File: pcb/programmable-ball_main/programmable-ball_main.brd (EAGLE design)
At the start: 30.5 x 30.8 mm, 2 parts, among them J1 USB4125-GF-A_REVA2, U1 MDBT50Q-1MV2

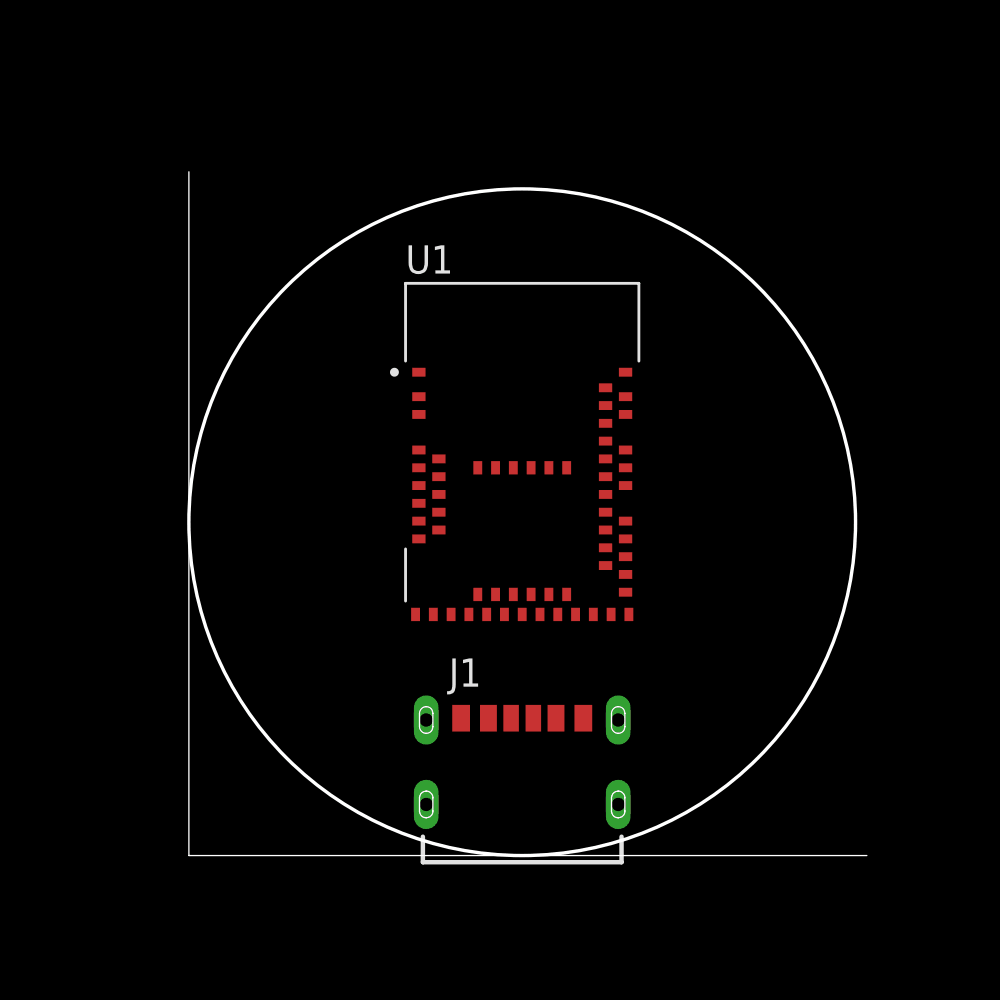
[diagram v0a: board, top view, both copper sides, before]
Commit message: 軽微な修正
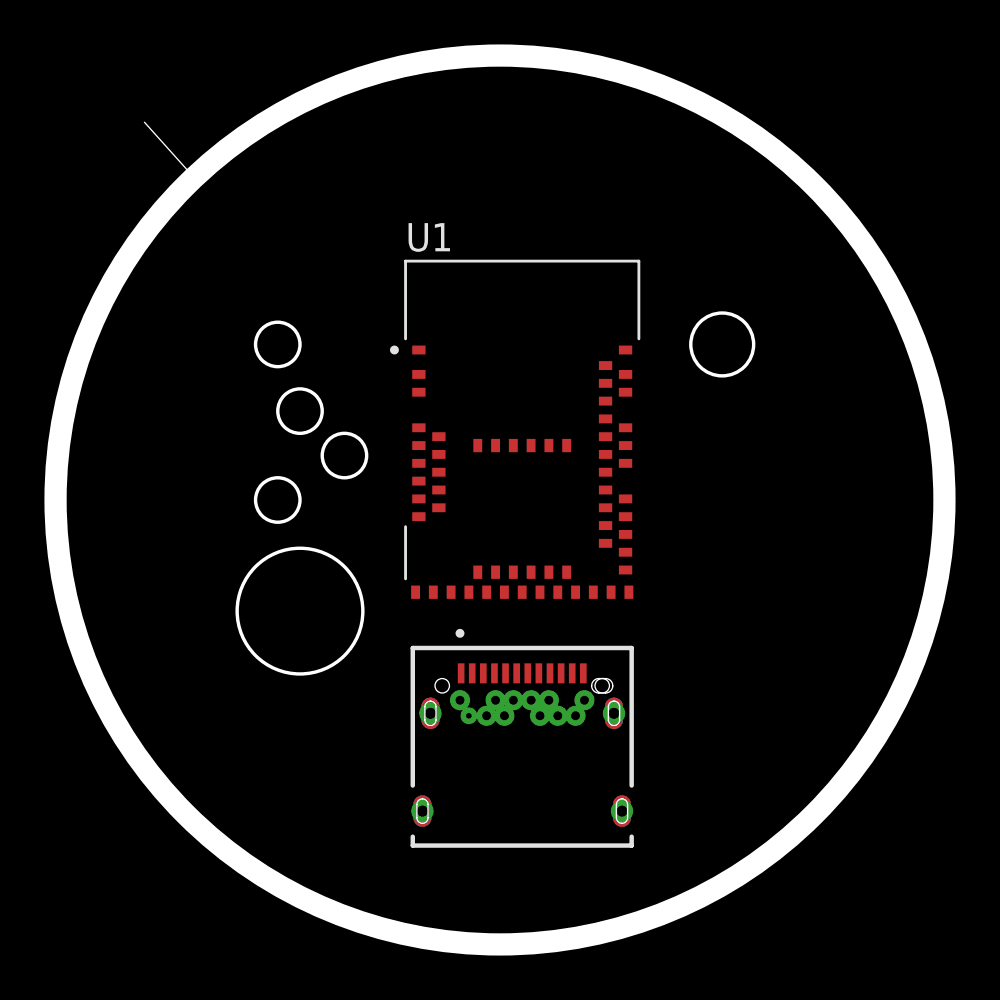
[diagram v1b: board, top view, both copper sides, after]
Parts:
- J1: value USB4125-GF-A_REVA2 -> USB4056-03-A_REVA2; device USB4125-GF-A_REVA2:GCT_USB4125-GF-A_REVA2 -> USB4056-03-A_REVA2:GCT_USB4056-03-A_REVA2
- moved J1 1.10 mm to (15.0, 2.00)
- moved U1 1.00 mm to (15.0, 19.0)
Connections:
- new net GND_A: J1.A1, J1.A12
- new net GND_B: J1.B1, J1.B12
- new net SHELL_GND: J1.S1, J1.S2, J1.S3, J1.S4
- new net USBD+: U1.35
- new net USBD-: U1.34
- new net VBUS_A: J1.A4, J1.A9
- new net VBUS_B: J1.B4, J1.B9
- net GND: no longer J1.A12, J1.B12
- net VBUS: no longer J1.A9, J1.B9
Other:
- board size 30.5 x 30.8 mm -> 40 x 40 mm
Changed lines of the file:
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@@
 <board>
 <plain>
-<wire x1="0" y1="0" x2="30.51" y2="0" width="0" layer="20"/>
-<wire x1="0" y1="30.77" x2="0" y2="0" width="0" layer="20"/>
+<wire x1="0" y1="30.77" x2="-2" y2="33" width="0" layer="20"/>
 <dimension x1="0" y1="0" x2="0" y2="30" x3="-6" y3="15" textsize="1.778" layer="47"/>
 <dimension x1="0" y1="0" x2="30" y2="0" x3="15" y3="-6" textsize="1.778" layer="47"/>
-<circle x="15" y="15" radius="15" width="0.1524" layer="20"/>
+<circle x="14" y="16" radius="20" width="1" layer="20"/>
+<circle x="4" y="16" radius="1" width="0.1524" layer="20"/>
+<circle x="5" y="11" radius="2.828425" width="0.1524" layer="20"/>
+<circle x="7" y="18" radius="1" width="0.1524" layer="20"/>
+<circle x="4" y="23" radius="1" width="0.1524" layer="20"/>
+<circle x="5" y="20" radius="1" width="0.1524" layer="20"/>
+<circle x="24" y="23" radius="1.4142125" width="0.1524" layer="20"/>
 </plain>
 <attributes>
@@
 </autorouter>
 <elements>
-<element name="U1" library="MDBT50Q-1MV2" package="XCVR_MDBT50Q-1MV2" value="MDBT50Q-1MV2" x="15" y="18" smashed="yes">
-<attribute name="AVAILABILITY" value="In Stock" x="15" y="18" size="1.778" layer="27" display="off"/>
-<attribute name="CHECK_PRICES" value="https://www.snapeda.com/parts/MDBT50Q-1MV2/Raytac+Corporation/view-part/?ref=eda" x="15" y="18" size="1.778" layer="27" display="off"/>
-<attribute name="DESCRIPTION" value=" 802.15.4, Bluetooth Bluetooth v5.2, Zigbee® Transceiver Module 2.36GHz ~ 2.5GHz Integrated, Chip Surface Mount " x="15" y="18" size="1.778" layer="27" display="off"/>
-<attribute name="MF" value="Raytac Corporation" x="15" y="18" size="1.778" layer="27" display="off"/>
-<attribute name="MP" value="MDBT50Q-1MV2" x="15" y="18" size="1.778" layer="27" display="off"/>
-<attribute name="NAME" x="9.75" y="26.19" size="1.27" layer="25"/>
-<attribute name="PACKAGE" value="SMD-61 Raytac Corporation" x="15" y="18" size="1.778" layer="27" display="off"/>
-<attribute name="PRICE" value="None" x="15" y="18" size="1.778" layer="27" display="off"/>
-<attribute name="SNAPEDA_LINK" value="https://www.snapeda.com/parts/MDBT50Q-1MV2/Raytac+Corporation/view-part/?ref=snap" x="15" y="18" size="1.778" layer="27" display="off"/>
+<element name="U1" library="MDBT50Q-1MV2" package="XCVR_MDBT50Q-1MV2" value="MDBT50Q-1MV2" x="15" y="19" smashed="yes">
+<attribute name="AVAILABILITY" value="In Stock" x="15" y="19" size="1.778" layer="27" display="off"/>
+<attribute name="CHECK_PRICES" value="https://www.snapeda.com/parts/MDBT50Q-1MV2/Raytac+Corporation/view-part/?ref=eda" x="15" y="19" size="1.778" layer="27" display="off"/>
+<attribute name="DESCRIPTION" value=" 802.15.4, Bluetooth Bluetooth v5.2, Zigbee® Transceiver Module 2.36GHz ~ 2.5GHz Integrated, Chip Surface Mount " x="15" y="19" size="1.778" layer="27" display="off"/>
+<attribute name="MF" value="Raytac Corporation" x="15" y="19" size="1.778" layer="27" display="off"/>
+<attribute name="MP" value="MDBT50Q-1MV2" x="15" y="19" size="1.778" layer="27" display="off"/>
+<attribute name="NAME" x="9.75" y="27.19" size="1.27" layer="25"/>
+<attribute name="PACKAGE" value="SMD-61 Raytac Corporation" x="15" y="19" size="1.778" layer="27" display="off"/>
+<attribute name="PRICE" value="None" x="15" y="19" size="1.778" layer="27" display="off"/>
+<attribute name="SNAPEDA_LINK" value="https://www.snapeda.com/parts/MDBT50Q-1MV2/Raytac+Corporation/view-part/?ref=snap" x="15" y="19" size="1.778" layer="27" display="off"/>
 </element>
-<element name="J1" library="USB4125-GF-A_REVA2" package="GCT_USB4125-GF-A_REVA2" value="USB4125-GF-A_REVA2" x="15" y="3.1" smashed="yes">
-<attribute name="DESCRIPTION" value=" USB Charge Only Connector Type C Horizontal Receptacle, 3.16mm profile, 6 Pins, Surface mount, Top mount, low cost " x="15" y="3.1" size="1.778" layer="27" display="off"/>
-<attribute name="DIGI-KEY_PART_NUMBER" value="2073-USB4125-GF-ATR-ND" x="15" y="3.1" size="1.778" layer="27" display="off"/>
-<attribute name="MF" value="Global Connector Technology" x="15" y="3.1" size="1.778" layer="27" display="off"/>
-<attribute name="MP" value="USB4125-GF-A" x="15" y="3.1" size="1.778" layer="27" display="off"/>
-<attribute name="NAME" x="11.7" y="7.6" size="1.27" layer="25"/>
-<attribute name="PACKAGE" value="None" x="15" y="3.1" size="1.778" layer="27" display="off"/>
-<attribute name="PURCHASE-URL" value="https://pricing.snapeda.com/search/part/USB4125-GF-A/?ref=eda" x="15" y="3.1" size="1.778" layer="27" display="off"/>
+<element name="J1" library="USB4056-03-A_REVA2" package="GCT_USB4056-03-A_REVA2" value="USB4056-03-A_REVA2" x="15" y="2" smashed="yes">
+<attribute name="AVAILABILITY" value="In Stock" x="15" y="2" size="1.778" layer="27" display="off"/>
+<attribute name="CHECK_PRICES" value="https://www.snapeda.com/parts/USB4056-03-A/Global+Connector+Technology/view-part/?ref=eda" x="15" y="2" size="1.778" layer="27" display="off"/>
+<attribute name="DESCRIPTION" value=" USB-C (USB TYPE-C) USB 3.2 Gen 2 (USB 3.1 Gen 2, Superspeed + (USB 3.1)) Receptacle Connector 24 Position Surface Mount, Right Angle; Through Hole " x="15" y="2" size="1.778" layer="27" display="off"/>
+<attribute name="MF" value="Global Connector Technology" x="15" y="2" size="1.778" layer="27" display="off"/>
+<attribute name="MP" value="USB4056-03-A" x="15" y="2" size="1.778" layer="27" display="off"/>
+<attribute name="PACKAGE" value="None" x="15" y="2" size="1.778" layer="27" display="off"/>
+<attribute name="PRICE" value="None" x="15" y="2" size="1.778" layer="27" display="off"/>
+<attribute name="SNAPEDA_LINK" value="https://www.snapeda.com/parts/USB4056-03-A/Global+Connector+Technology/view-part/?ref=snap" x="15" y="2" size="1.778" layer="27" display="off"/>
 </element>
 </elements>
@@
 <contactref element="U1" pad="33"/>
 <contactref element="U1" pad="2"/>
-<contactref element="J1" pad="B12"/>
-<contactref element="J1" pad="A12"/>
-<wire x1="10.35" y1="21.75" x2="19.65" y2="21.75" width="0" layer="19" extent="1-1"/>
-<wire x1="10.35" y1="20.65" x2="10.35" y2="21.75" width="0" layer="19" extent="1-1"/>
-<wire x1="10.2" y1="10.85" x2="10.35" y2="20.65" width="0" layer="19" extent="1-1"/>
-<wire x1="19.8" y1="10.85" x2="10.2" y2="10.85" width="0" layer="19" extent="1-1"/>
-<wire x1="17.75" y1="6.18" x2="10.2" y2="10.85" width="0" layer="19" extent="1-1"/>
-<wire x1="12.25" y1="6.18" x2="17.75" y2="6.18" width="0" layer="19" extent="1-1"/>
+<wire x1="10.35" y1="22.75" x2="19.65" y2="22.75" width="0" layer="19" extent="1-1"/>
+<wire x1="10.35" y1="21.65" x2="10.35" y2="22.75" width="0" layer="19" extent="1-1"/>
+<wire x1="10.2" y1="11.85" x2="10.35" y2="21.65" width="0" layer="19" extent="1-1"/>
+<wire x1="19.8" y1="11.85" x2="10.2" y2="11.85" width="0" layer="19" extent="1-1"/>
 </signal>
 <signal name="VDDH">
@@
 <signal name="VBUS">
 <contactref element="U1" pad="32"/>
-<contactref element="J1" pad="B9"/>
-<contactref element="J1" pad="A9"/>
-<wire x1="16.52" y1="6.18" x2="19" y2="10.85" width="0" layer="19" extent="1-1"/>
-<wire x1="13.48" y1="6.18" x2="16.52" y2="6.18" width="0" layer="19" extent="1-1"/>
 </signal>
 <signal name="DCCH">
@@
 <contactref element="U1" pad="28"/>
 </signal>
+<signal name="USBD+">
+<contactref element="U1" pad="35"/>
+</signal>
+<signal name="USBD-">
+<contactref element="U1" pad="34"/>
+</signal>
+<signal name="GND_A">
+<contactref element="J1" pad="A12"/>
+<contactref element="J1" pad="A1"/>
+<wire x1="17.75" y1="8.2" x2="12.25" y2="8.2" width="0" layer="19" extent="1-1"/>
+</signal>
+<signal name="VBUS_A">
+<contactref element="J1" pad="A4"/>
+<contactref element="J1" pad="A9"/>
+<wire x1="16.25" y1="8.2" x2="13.75" y2="8.2" width="0" layer="19" extent="1-1"/>
+</signal>
+<signal name="SHELL_GND">
+<contactref element="J1" pad="S2"/>
+<contactref element="J1" pad="S1"/>
+<contactref element="J1" pad="S4"/>
+<contactref element="J1" pad="S3"/>
+<wire x1="10.87" y1="6.4" x2="10.51" y2="2" width="0" layer="19" extent="1-1"/>
+<wire x1="19.13" y1="6.4" x2="10.87" y2="6.4" width="0" layer="19" extent="1-1"/>
+<wire x1="19.49" y1="2" x2="19.13" y2="6.4" width="0" layer="19" extent="1-1"/>
+</signal>
+<signal name="GND_B">
+<contactref element="J1" pad="B12"/>
+<contactref element="J1" pad="B1"/>
+<wire x1="17.8" y1="6.99" x2="12.2" y2="6.99" width="0" layer="19" extent="1-1"/>
+</signal>
+<signal name="VBUS_B">
+<contactref element="J1" pad="B9"/>
+<contactref element="J1" pad="B4"/>
+<wire x1="16.2" y1="6.99" x2="13.8" y2="6.99" width="0" layer="19" extent="1-1"/>
+</signal>
 </signals>

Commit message: usb typeC周り実装 #4
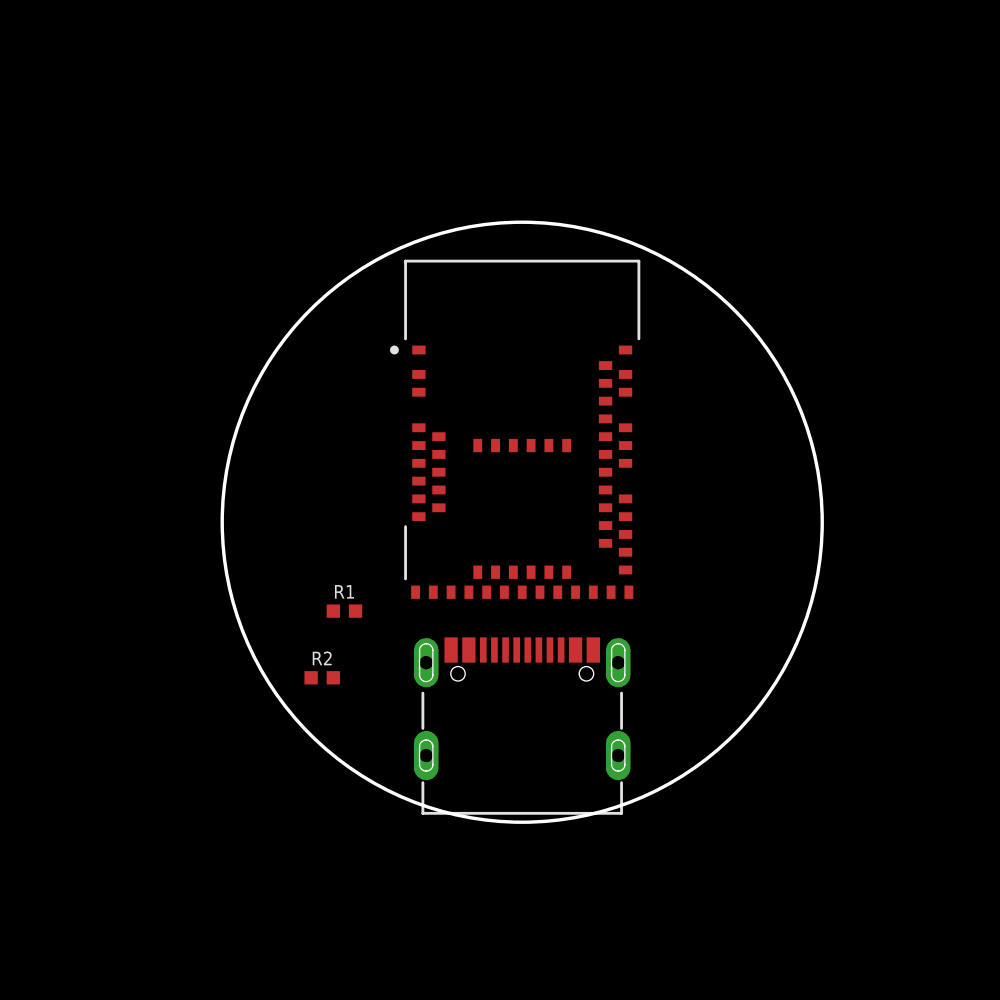
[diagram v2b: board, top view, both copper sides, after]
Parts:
- added R1, R2: 5.1k, SparkFun-Resistors:0402-TIGHT
- J1: value USB4056-03-A_REVA2 -> 12402012E212A; device USB4056-03-A_REVA2:GCT_USB4056-03-A_REVA2 -> 12402012E212A:AMPHENOL_12402012E212A
- moved J1 2.50 mm to (15.0, 4.50)
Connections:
- removed net GND_A: J1.A1, J1.A12
- removed net GND_B: J1.B1, J1.B12
- removed net SHELL_GND: J1.S1, J1.S2, J1.S3, J1.S4
- removed net VBUS_A: J1.A4, J1.A9
- removed net VBUS_B: J1.B4, J1.B9
- new net N$1: J1.A5, R1.2
- new net N$2: J1.B5, R2.2
- net GND: now also J1.A1_B12, J1.B1_A12, R1.1, R2.1
- net USBD+: now also J1.A6, J1.B6
- net USBD-: now also J1.A7, J1.B7
- net VBUS: now also J1.A4_B9, J1.B4_A9
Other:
- board size 40 x 40 mm -> 27 x 27 mm
